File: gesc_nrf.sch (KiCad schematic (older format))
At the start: 5 parts, among them J14 Conn_01x03, U16 EYSGJNZWY

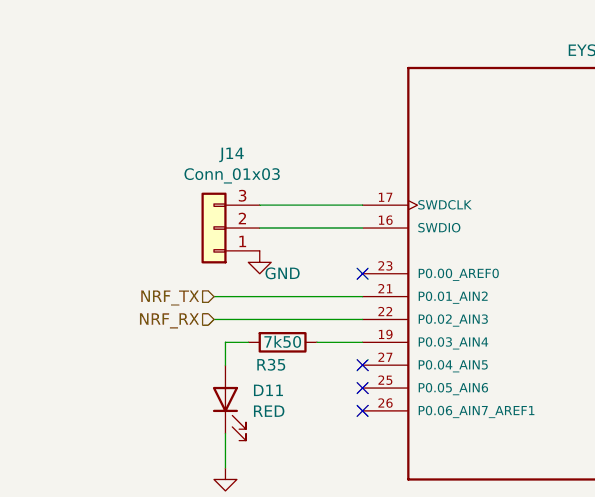
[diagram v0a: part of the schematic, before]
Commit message: save
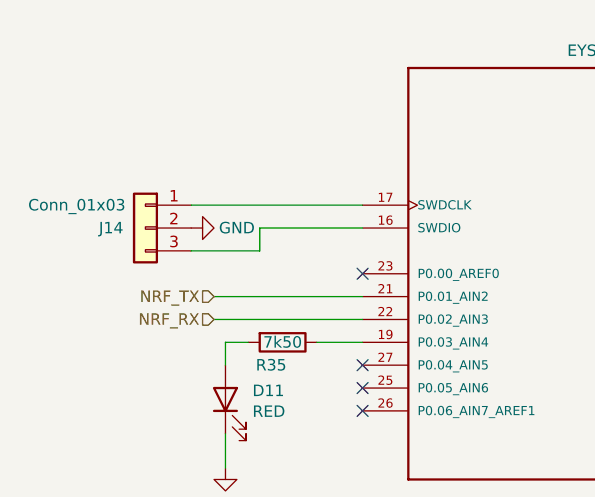
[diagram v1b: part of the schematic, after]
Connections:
- net GND: now also J14.2 (Pin_2); no longer J14.1 (Pin_1)
- net at U16.16 (SWDIO): now also J14.3 (Pin_3); no longer J14.2 (Pin_2)
- net at U16.17 (SWDCLK): now also J14.1 (Pin_1); no longer J14.3 (Pin_3)
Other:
- moved on the sheet: J14
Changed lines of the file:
@@
 L Connector_Generic:Conn_01x03 J14
 U 1 1 5E9FAF5C
-P 3350 4350
-F 0 "J14" H 3270 4025 50  0000 C CNN
-F 1 "Conn_01x03" H 3270 4116 50  0000 C CNN
-F 2 "Connector_PinHeader_2.54mm:PinHeader_1x03_P2.54mm_Vertical" H 3350 4350 50  0001 C CNN
-F 3 "~" H 3350 4350 50  0001 C CNN
-	1    3350 4350
-	-1   0    0    1
+P 3050 4350
+F 0 "J14" H 3200 4350 50  0000 C CNN
+F 1 "Conn_01x03" H 3350 4450 50  0000 C CNN
+F 2 "Connector_PinHeader_2.54mm:PinHeader_1x03_P2.54mm_Vertical" H 3050 4350 50  0001 C CNN
+F 3 "~" H 3050 4350 50  0001 C CNN
+	1    3050 4350
+	-1   0    0    -1
 $EndComp
 Wire Wire Line
 	4000 4350 3550 4350
-Wire Wire Line
-	3550 4250 4000 4250
 $Comp
 L power:GND #PWR0158
 U 1 1 5E9FB3BA
-P 3550 4450
-F 0 "#PWR0158" H 3550 4200 50  0001 C CNN
-F 1 "GND" H 3650 4350 50  0000 C CNN
-F 2 "" H 3550 4450 50  0001 C CNN
-F 3 "" H 3550 4450 50  0001 C CNN
-	1    3550 4450
-	1    0    0    -1
+P 3250 4350
+F 0 "#PWR0158" H 3250 4100 50  0001 C CNN
+F 1 "GND" V 3250 4150 50  0000 C CNN
+F 2 "" H 3250 4350 50  0001 C CNN
+F 3 "" H 3250 4350 50  0001 C CNN
+	1    3250 4350
+	0    -1   -1   0
 $EndComp
+Wire Wire Line
+	3250 4250 4000 4250
+Wire Wire Line
+	3550 4350 3550 4450
+Wire Wire Line
+	3550 4450 3250 4450
 $EndSCHEMATC
